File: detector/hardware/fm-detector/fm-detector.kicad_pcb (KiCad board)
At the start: 2 copper layers, 50 x 50 mm, 116 parts, among them J1 JST PH, J2 U.FL, J3 U.FL, J4 3.5mm audio socket, J5 U.FL, J6 U.FL, J7 U.FL, J8 SMA-RA, Q1 MMBT3904, Q10 MMBT3904, Q11 MMBT3904, Q2 MMBT3904, Q3 BSS138, Q4 MMBT3904, Q5 MMBT3904, Q6 MMBT3904, Q7 MMBT3904, Q8 MMBT3904, Q9 MMBT3904, Y1 10.7M

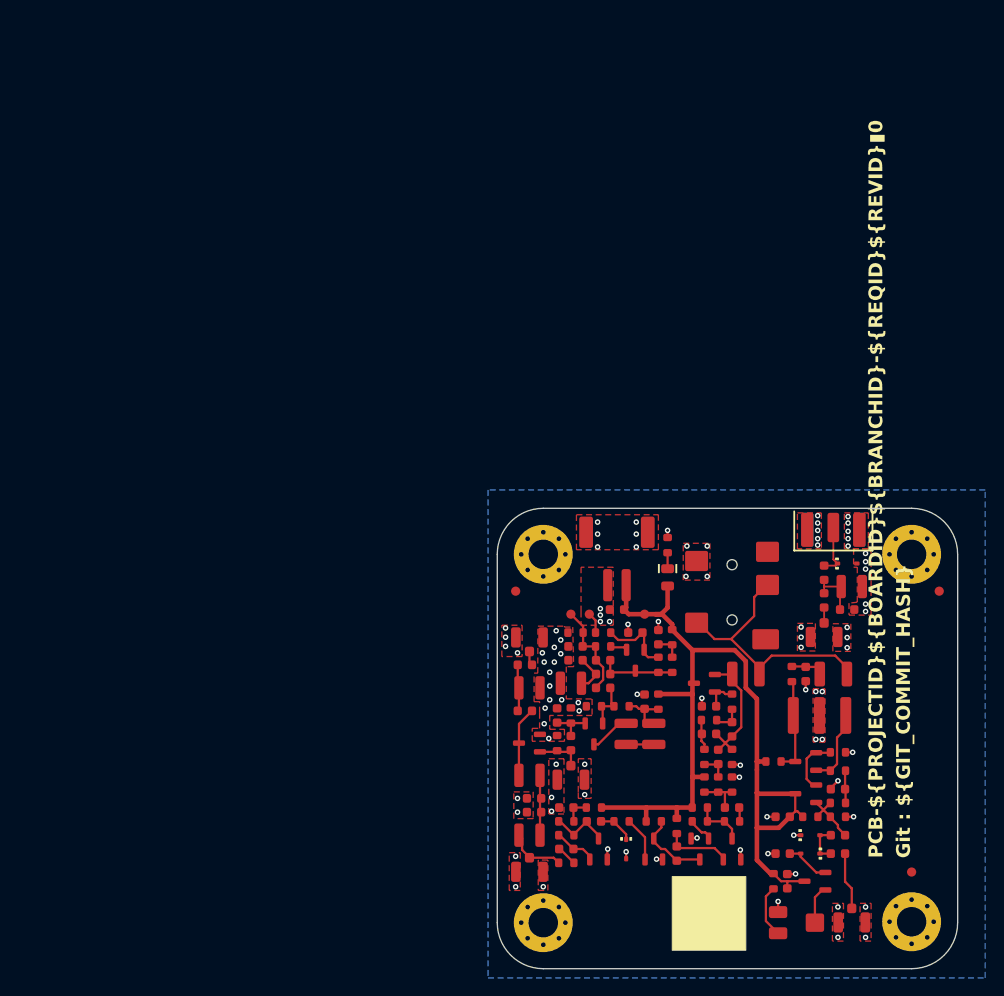
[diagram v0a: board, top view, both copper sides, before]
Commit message: PCB-0010-0100 ready for release
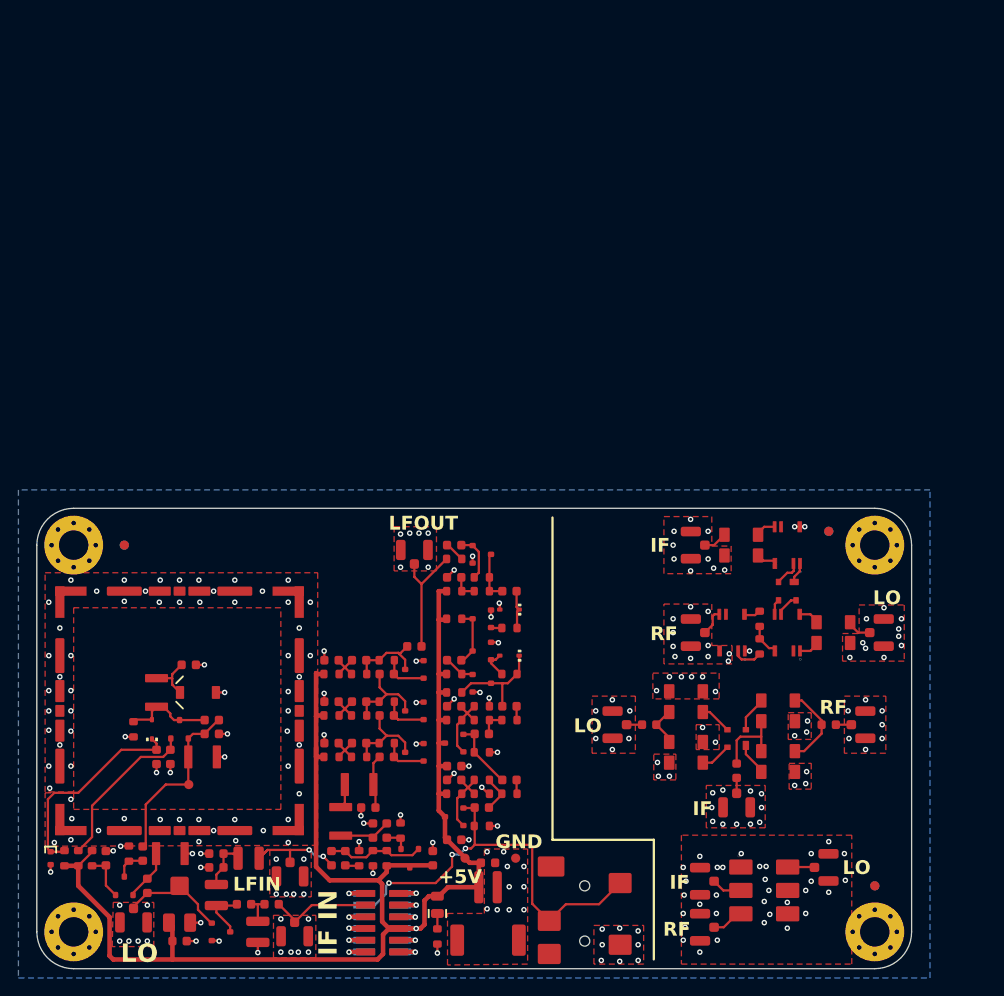
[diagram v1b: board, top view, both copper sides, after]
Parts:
- removed D5: 3V3, g-dio:D_SOD-323
- removed L7: 180n, g-ind:L_Coilcraft_1008HQ_2520Metric
- removed R36: 8K2, g-res:R_0603_1608Metric
- removed R37: 10K, g-res:R_0603_1608Metric
- removed Y1: 10.7M, g-fil:Resonator_SMD_Murata_SFECV-3Pin_6.9x2.9mm
- added C37: 2p - 6p, g-cap:C_Trimmer_Voltronics_JZ, F.Cu at (48.5, 54.0)
- added C38: 180p, g-cap:C_0603_1608Metric, F.Cu at (50.0, 57.0)
- added C39: 180p, g-cap:C_0603_1608Metric, F.Cu at (50.0, 58.5)
- added C40: 47p, g-cap:C_0603_1608Metric, F.Cu at (47.5, 51.0)
- added C41: 100n, g-cap:C_0603_1608Metric, F.Cu at (45.5, 61.0)
- added C42: 2p, g-cap:C_0603_1608Metric, F.Cu at (42.5, 71.5)
- added C43: 100n, g-cap:C_0603_1608Metric, F.Cu at (44.0, 61.0)
- added C44: 100n, g-cap:C_0603_1608Metric, F.Cu at (38.5, 72.0)
- added C45: 100n, g-cap:C_0603_1608Metric, F.Cu at (43.0, 75.0)
- added C46: 10n, g-cap:C_0603_1608Metric, F.Cu at (107.0, 62.5)
- added D6: 1N4148, g-dio:D_SOD-323, F.Cu at (43.5, 58.0)
- added D7: 3V0, g-dio:D_SOD-523, F.Cu at (32.5, 72.0)
- added D8: 1N4148, g-dio:D_SOD-323, F.Cu at (82.3, 50.0)
- added FD4: Fiducial, g-no_bom:Fiducial_1mm_Mask2mm, B.Cu at (40.5, 38.0)
- added FD5: Fiducial, g-no_bom:Fiducial_1mm_Mask2mm, B.Cu at (117.0, 36.5)
- added FD6: Fiducial, g-no_bom:Fiducial_1mm_Mask2mm, B.Cu at (122.0, 75.0)
- added FL1: 22µ, g-fil:L_Wurth_WE-CNSW-1812, F.Cu at (117.5, 47.5)
- added FL2: 22µ, g-fil:L_Wurth_WE-CNSW-1812, F.Cu at (101.5, 55.0)
- added FL3: 22µ, g-fil:L_Wurth_WE-CNSW-1812, F.Cu at (107.5, 38.0)
- added FL4: 22µ, g-fil:L_Wurth_WE-CNSW-1812, F.Cu at (111.5, 61.5)
- added FL5: 22µ, g-fil:L_Wurth_WE-CNSW-1812, F.Cu at (101.5, 60.5)
- added FL6: 22µ, g-fil:L_Wurth_WE-CNSW-1812, F.Cu at (111.5, 56.0)
- added H10: S0991-46R, g-rfm:H_Harwin_S0991-46R, F.Cu at (46.5, 69.0)
- added H5: S0991-46R, g-rfm:H_Harwin_S0991-46R, F.Cu at (33.5, 56.0)
- added H7: S0991-46R, g-rfm:H_Harwin_S0991-46R, F.Cu at (46.5, 43.0)
- added H9: S0991-46R, g-rfm:H_Harwin_S0991-46R, F.Cu at (59.5, 56.0)
- added J10: U.FL, g-con:U.FL_Hirose_U.FL-R-SMT-1_Vertical, F.Cu at (102.5, 38.0)
- added J11: 2x06M, g-con:PinHeader_2x06_P1.27mm_Vertical_SMD, B.Cu at (68.5, 79.0)
- added J12: 2x06F, g-con:PinSocket_2x06_P1.27mm_Vertical_SMD, F.Cu at (68.5, 79.0)
- added J13: U.FL, g-con:U.FL_Hirose_U.FL-R-SMT-1_Vertical, F.Cu at (94.0, 57.5)
- added J14: U.FL, g-con:U.FL_Hirose_U.FL-R-SMT-1_Vertical, F.Cu at (107.0, 66.0)
- added J15: U.FL, g-con:U.FL_Hirose_U.FL-R-SMT-1_Vertical, F.Cu at (120.5, 57.5)
- added J16: U.FL, g-con:U.FL_Hirose_U.FL-R-SMT-1_Vertical, F.Cu at (103.5, 79.5)
- added J17: U.FL, g-con:U.FL_Hirose_U.FL-R-SMT-1_Vertical, F.Cu at (103.5, 74.5)
- added J18: U.FL, g-con:U.FL_Hirose_U.FL-R-SMT-1_Vertical, F.Cu at (116.5, 73.0)
- added J9: U.FL, g-con:U.FL_Hirose_U.FL-R-SMT-1_Vertical, F.Cu at (102.5, 47.5)
- added L8: 47µ, g-ind:L_Murata_LQW32FT_3225, F.Cu at (49.0, 61.0)
- added L9: 47µ, g-ind:L_Murata_LQW32FT_3225, F.Cu at (45.5, 71.5)
- added Q12: J309, g-SOT:SOT-23-3, F.Cu at (46.5, 58.0)
- added Q13: J309, g-SOT:SOT-23-3, F.Cu at (40.5, 75.0)
- added R38: 100K, g-res:R_0603_1608Metric, F.Cu at (41.5, 58.0)
- added R39: 47E, g-res:R_0603_1608Metric, F.Cu at (35.5, 72.0)
- added R40: 1K, g-res:R_0603_1608Metric, F.Cu at (34.0, 72.0)
- added R41: 100K, g-res:R_0603_1608Metric, F.Cu at (41.0, 71.5)
- added R42: 47E, g-res:R_0603_1608Metric, F.Cu at (37.0, 72.0)
- added T1: 240µ, g-ind:T_Wurth_WE-STST-4532_74930000, F.Cu at (112.5, 47.5)
- added T2: 240µ, g-ind:T_Wurth_WE-STST-4532_74930000, F.Cu at (112.5, 38.0)
- added T3: 240µ, g-ind:T_Wurth_WE-STST-4532_74930000, F.Cu at (106.5, 47.5)
- added U1: ADE-1+, g-rfm:H_Mini-Circuits_CD636_H4.11mm, F.Cu at (110.0, 75.5)
- C1, C10, C2, C24, C27, C31: value 10n -> 100n
- C18: value 330p -> 150p
- C19: value 10µ -> 150p; footprint g-cap:C_1210_3225Metric -> g-cap:C_0603_1608Metric
- C20: value 470n -> 100n
- C21, C23: value 390p -> 100n
- C22: value 390p -> 150p
- C26, C5: value 220p -> 100n
- C28: value 10n -> 1.5n
- C29, C33: value 10n -> 820p
- C3: value 18p -> 100n
- C30: value 10µ -> 100n; footprint g-cap:C_1210_3225Metric -> g-cap:C_0603_1608Metric
- C32: value 220p -> 1.5n
- C34: value 10p -> 100n
- C35: value 10p -> 10n
- C36: value 4p -> 10n
- C4: value 18p -> 4.7n
- C6: value 10n -> 12n
- C8: value 10p -> 150p
- C9: value 82p -> 100n
- D3, D4: value 1N4148 -> BAT15-099R; footprint g-dio:D_SOD-323 -> g-SOT:SOT-143
- J6: value U.FL -> 2118708-2; footprint g-con:U.FL_Hirose_U.FL-R-SMT-1_Vertical -> g-rfm:H_TE_2118708
- J8: value SMA-RA -> U.FL; footprint g-con:SMA_Samtec_SMA-J-P-H-ST-EM1_EdgeMount -> g-con:U.FL_Hirose_U.FL-R-SMT-1_Vertical
- L1: footprint g-ind:L_Coilcraft_1008HQ_2520Metric -> g-ind:L_Murata_LQW32FT_3225
- L2, L3: value 6µ8 -> 18µ; footprint g-ind:L_Coilcraft_1008HQ_2520Metric -> g-ind:L_Murata_LQW32FT_3225
- R1: value 100E -> 51E
- R10: value 1K5 -> 150K
- R12: value 100E -> 3K9
- R2: value 4K7 -> 3K6
- R21: value 20K -> 10K
- R22: value 0E -> 1M
- R23: value 470K -> 100E
- R24: value 470K -> 3K9
- R25: value 15K -> 39K
- R26: value 15K -> 3K3
- R28: value 8K2 -> 10K
- R29: value 2K2 -> 15K
- R3: value 2K2 -> 1K5
- R30: value 13K -> 3K3
- R31: value 12K -> 39K
- R32: value 22K -> 150K
- R33: value 5K6 -> 10K
- R34: value 1K -> 0E
- R35: value 47K -> 0E
- R4: value 100E -> 1K2
- R5: value 1K2 -> 1M
- R6: value 22K -> 100E
- R7: value 4K7 -> 3K9
- R8: value 1K8 -> 1M
- moved FD3 88.6 mm to (40.5, 38.0)
- moved J8 87.0 mm to (41.5, 78.5), turned to -90 degrees
- moved J6 76.4 mm to (46.5, 56.0)
- moved C26 72.4 mm to (46.5, 81.0)
- moved RV1 67.0 mm to (46.5, 77.0), turned to 180 degrees
- moved H1 51.0 mm to (35.0, 80.0)
- moved H2 51.0 mm to (35.0, 38.0)
- moved FD1 50.4 mm to (122.0, 75.0)
- moved C34 49.5 mm to (76.3, 70.0), turned to 180 degrees
- moved J4 49.5 mm to (90.5, 84.0), turned to 180 degrees
- moved R11 49.3 mm to (74.5, 80.5), turned to 90 degrees
- moved TP3 45.4 mm to (47.5, 64.0), turned to 90 degrees
- moved L1 45.0 mm to (44.0, 54.0), turned to -90 degrees
- moved C23 44.1 mm to (63.0, 50.5), turned to 180 degrees
- moved C20 44.1 mm to (63.0, 59.5)
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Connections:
- net /Mixer/IF renamed /IF
- C1 pad 1: GND -> Net-(C1-Pad1)
- C1 pad 2: Net-(C1-Pad2) -> Net-(Q1-B)
- C10 pad 1: GND -> /IF2_amp/IF2_amp_stage_I/IN
- C10 pad 2: Net-(C10-Pad2) -> Net-(Q8-B)
- C19 pad 1: Net-(Q8-E) -> /IF2_amp/IF2_amp_stage_I/OUT
- C19 pad 2: /Detector/AF -> Net-(C19-Pad2)
- C2 pad 1: GND -> /LFIN
- C20 pad 1: Net-(C20-Pad1) -> Net-(C19-Pad2)
- C20 pad 2: Net-(C20-Pad2) -> GND
- C21 pad 1: Net-(Q8-E) -> /IF2_amp/IF2_amp_stage_II/OUT
- C21 pad 2: Net-(C21-Pad2) -> Net-(Q10-B)
- C22 pad 1: Net-(Q8-E) -> /IF2_amp/IF2_amp_stage_III/OUT
- C23 pad 1: Net-(Q8-E) -> Net-(C22-Pad2)
- C23 pad 2: Net-(C23-Pad2) -> GND
- C24 pad 1: GND -> /IF2_amp/IF2_amp_stage_III/OUT
- C24 pad 2: Net-(Q8-B) -> /LFOUT
- C26 pad 1: Net-(D3-A) -> +5V
- C26 pad 2: Net-(Q9-B) -> GND
- C27 pad 1: GND -> /PPM
- C28 pad 1: GND -> /audio filter 1/OUT
- C28 pad 2: +5V -> Net-(C28-Pad2)
- C29 pad 2: Net-(C29-Pad2) -> Net-(Q9-B)
- C3 pad 1: Net-(Q1-C) -> Net-(Q1-E)
- C30 pad 1: Net-(C29-Pad2) -> GND
- C30 pad 2: /Detector/AF -> +5V
- C31 pad 1: GND -> /audio filter 1/OUT
- C31 pad 2: Net-(D4-A) -> Net-(C31-Pad2)
- C32 pad 1: Net-(J6-In) -> /AUDIO
- C32 pad 2: Net-(D3-A) -> Net-(C32-Pad2)
- C33 pad 2: +5V -> Net-(Q11-B)
- C34 pad 1: Net-(D5-CH1) -> GND
- C34 pad 2: Net-(C34-Pad2) -> +5V
- C35 pad 1: Net-(C34-Pad2) -> /DBM Experiments/Diode Ring Mixer Transmission Line/LO
- C35 pad 2: Net-(J7-In) -> Net-(C35-Pad2)
- C36 pad 1: GND -> Net-(C36-Pad1)
- C36 pad 2: Net-(C34-Pad2) -> /DBM Experiments/Diode Ring Mixer Transmission Line/RF
- C5 pad 2: /Local Oscillator/OSC-OUT -> +5V
- C6 pad 2: Net-(Q2-E) -> /IF2_amp/IF2_amp_stage_I/IN
- C7 pad 1: Net-(Q2-E) -> /IF2_amp/IF2_amp_stage_I/OUT
- C7 pad 2: /Local Oscillator/LO -> Net-(Q2-B)
- C8 pad 1: /Local Oscillator/OSC-OUT -> /IF2_amp/IF2_amp_stage_II/OUT
- C8 pad 2: Net-(Q2-B) -> Net-(C8-Pad2)
- C9 pad 1: /Local Oscillator/OSC-OUT -> Net-(C8-Pad2)
- C9 pad 2: Net-(Q1-C) -> GND
- D3 pad 1: GND -> Net-(D3-Pad1)
- D3 pad 2: Net-(D3-A) -> Net-(D3-Pad2)
- D4 pad 1: Net-(D3-A) -> Net-(D4-Pad1)
- D4 pad 2: Net-(D4-A) -> Net-(D4-Pad2)
- J3 pad 1: /Detector/LF -> /LFIN
- J4 pad R: /Detector/AF -> /AUDIO
- J4 pad T: /Detector/AF -> /AUDIO
- J5 pad 1: /Local Oscillator/LO -> /LFOUT
- J6 pad 1: Net-(J6-In) -> GND
- J7 pad 1: Net-(J7-In) -> /DBM Experiments/Diode Ring Mixer/LO
- J8 pad 1: Net-(D5-CH1) -> /LO
- L1 pad 1: GND -> Net-(C37-Pad1)
- L1 pad 2: Net-(C3-Pad2) -> Net-(D6-A)
- L2 pad 1: Net-(Q2-C) -> Net-(C3-Pad2)
- L3 pad 2: Net-(C10-Pad2) -> /IF2_amp/IF2_amp_stage_I/IN
- L6 pad 2: /Detector/LF -> /LFIN
- Q1 pad 3: Net-(Q1-C) -> +5V
- Q10 pad 2: Net-(Q10-E) -> GND
- Q10 pad 3: Net-(Q10-C) -> /IF2_amp/IF2_amp_stage_III/OUT
- Q11 pad 2: Net-(D4-A) -> /AUDIO
- Q2 pad 2: Net-(Q2-E) -> GND
- Q2 pad 3: Net-(Q2-C) -> /IF2_amp/IF2_amp_stage_II/OUT
- Q3 pad 1: /Local Oscillator/LO -> /LO
- Q7 pad 3: /Detector/PWM_AUDIO -> /PPM
- Q8 pad 2: Net-(Q8-E) -> GND
- Q8 pad 3: +5V -> /IF2_amp/IF2_amp_stage_I/OUT
- Q9 pad 2: Net-(Q10-E) -> /audio filter 1/OUT
- R1 pad 1: /Local Oscillator/OSC-OUT -> GND
- R1 pad 2: Net-(Q1-E) -> Net-(C1-Pad1)
- R10 pad 2: /Local Oscillator/LO -> Net-(Q9-B)
- R12 pad 1: Net-(C10-Pad2) -> /IF2_amp/IF2_amp_stage_I/OUT
- R12 pad 2: +5V -> Net-(C19-Pad2)
- R13 pad 1: /Detector/LF -> /LFOUT
- R2 pad 2: Net-(Q1-C) -> +5V
- R20 pad 1: /Detector/PWM_AUDIO -> /PPM
- R21 pad 2: /Detector/PWM_AUDIO -> /PPM
- R22 pad 1: /Detector/PWM_AUDIO -> Net-(Q10-B)
- R22 pad 2: Net-(C20-Pad1) -> /IF2_amp/IF2_amp_stage_III/OUT
- R23 pad 1: Net-(C20-Pad2) -> Net-(C22-Pad2)
- R24 pad 1: GND -> /IF2_amp/IF2_amp_stage_III/OUT
- R24 pad 2: Net-(C20-Pad2) -> Net-(C22-Pad2)
- R25 pad 1: Net-(C20-Pad2) -> Net-(Q9-B)
- R25 pad 2: Net-(C21-Pad2) -> +5V
- R26 pad 1: Net-(C21-Pad2) -> Net-(C28-Pad2)
- R26 pad 2: Net-(C22-Pad2) -> Net-(Q9-B)
- R27 pad 1: Net-(C22-Pad2) -> Net-(C27-Pad2)
- R27 pad 2: Net-(C23-Pad2) -> Net-(C28-Pad2)
- R28 pad 1: Net-(C23-Pad2) -> GND
- R28 pad 2: Net-(Q8-B) -> /audio filter 1/OUT
- R29 pad 1: GND -> Net-(C31-Pad2)
- R29 pad 2: Net-(Q8-E) -> Net-(C32-Pad2)
- R3 pad 1: Net-(Q1-C) -> GND
- R3 pad 2: Net-(C1-Pad2) -> Net-(Q1-B)
- R30 pad 1: Net-(Q9-B) -> Net-(C32-Pad2)
- R30 pad 2: +5V -> Net-(Q11-B)
- R31 pad 1: GND -> Net-(Q11-B)
- R31 pad 2: Net-(Q9-B) -> +5V
- R32 pad 1: Net-(Q9-B) -> GND
- R32 pad 2: Net-(C27-Pad2) -> Net-(Q11-B)
- R33 pad 1: Net-(Q10-C) -> GND
- R33 pad 2: +5V -> /AUDIO
- R34 pad 1: GND -> Net-(R34-Pad1)
- R34 pad 2: Net-(Q10-E) -> Net-(R34-Pad2)
- R35 pad 1: Net-(C27-Pad2) -> Net-(R35-Pad1)
- R35 pad 2: Net-(Q10-B) -> Net-(R34-Pad2)
- R4 pad 1: Net-(C1-Pad2) -> GND
- R4 pad 2: +5V -> Net-(Q1-E)
- R5 pad 1: GND -> Net-(Q2-B)
- R5 pad 2: /Local Oscillator/OSC-OUT -> /IF2_amp/IF2_amp_stage_II/OUT
- R6 pad 1: GND -> Net-(C8-Pad2)
- R6 pad 2: Net-(Q1-B) -> +5V
- R7 pad 1: Net-(Q2-B) -> /IF2_amp/IF2_amp_stage_II/OUT
- R7 pad 2: Net-(C10-Pad2) -> Net-(C8-Pad2)
- R8 pad 1: GND -> Net-(Q8-B)
- R8 pad 2: Net-(Q2-B) -> /IF2_amp/IF2_amp_stage_I/OUT
- R9 pad 1: GND -> Net-(C19-Pad2)
- R9 pad 2: Net-(Q2-E) -> +5V
- RV1 pad 1: GND -> +5V
- RV1 pad 2: Net-(Q11-B) -> /LO
- RV1 pad 3: Net-(R37-Pad1) -> GND
- TP3 pad 1: /Local Oscillator/OSC-OUT -> Net-(Q12-S)
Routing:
- net +5V: track 99.3 -> 153.1 mm, vias 0 -> 1
- net /AUDIO: track 0.00 -> 45.8 mm, vias 0 -> 3
- net GND: track 21.0 -> 51.4 mm, vias 94 -> 255
- net /Detector/AF: track 29.1 -> 0.00 mm
- net Net-(D6-K): track 0.00 -> 22.8 mm
- net Net-(Q12-S): track 0.00 -> 19.6 mm
- net Net-(Q12-D): track 0.00 -> 17.8 mm
- net Net-(Q8-E): track 14.3 -> 0.00 mm
- net /LFOUT: track 0.00 -> 13.1 mm
- net /LO: track 0.00 -> 12.2 mm
- net /LFIN: track 0.00 -> 11.4 mm, vias 0 -> 2
- net /PPM: track 0.00 -> 11.4 mm
- net /Local Oscillator/OSC-OUT: track 10.6 -> 0.00 mm
- net Net-(Q10-C): track 10.4 -> 0.00 mm
- net /IF2_amp/IF2_amp_stage_I/OUT: track 0.00 -> 9.95 mm
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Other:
- board size 50 x 50 mm -> 95 x 50 mm
- board text added: "+5V"
- board text added: "GND"
- board text added: "IF"
- board text added: "IF IN"
- board text added: "LFIN"
- board text added: "LFOUT"
- board text added: "LO"
- board text added: "RF"
